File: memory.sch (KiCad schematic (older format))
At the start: 9 parts, among them U5 IS42S16400J-xC

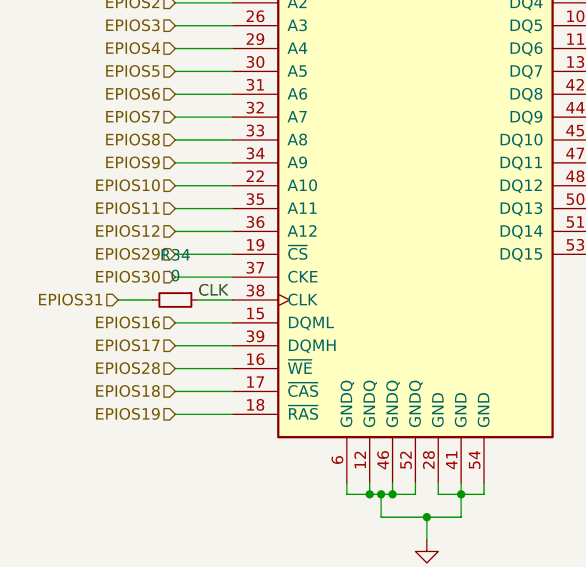
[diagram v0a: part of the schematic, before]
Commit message: updates
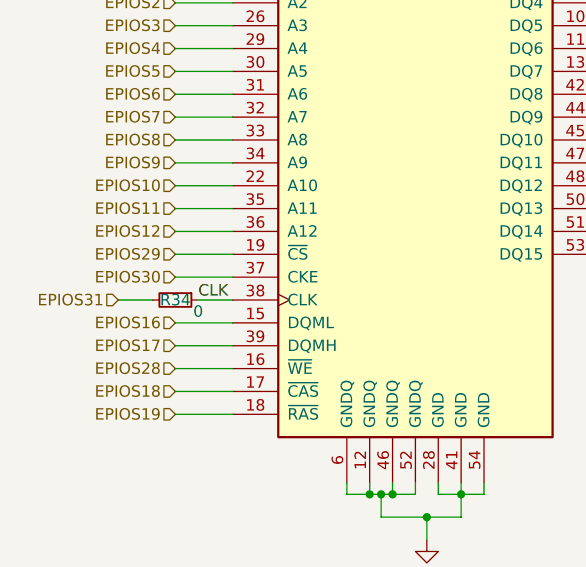
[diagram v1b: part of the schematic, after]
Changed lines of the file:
@@
 EESchema Schematic File Version 4
+LIBS:Raptor2000-cache
 EELAYER 29 0
 EELAYER END
 $Descr A4 11693 8268
 encoding utf-8
-Sheet 10 4
+Sheet 4 4
 Title ""
 Date ""
@@
 U 1 1 5CAC59FE
 P 4750 4050
-F 0 "R34" V 4554 4050 50  0000 C CNN
-F 1 "0" V 4645 4050 50  0000 C CNN
+F 0 "R34" V 4750 4050 50  0000 C CNN
+F 1 "0" V 4800 4150 50  0000 C CNN
 F 2 "Resistor_SMD:R_0603_1608Metric" H 4750 4050 50  0001 C CNN
 F 3 "~" H 4750 4050 50  0001 C CNN

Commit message: added nand flash, removed sd card. finished rtc circuit. added leds
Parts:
- added C14: 0.1, symbol Device:C
- added R4: 10k, symbol Device:R_Small
- added U3: TC58CVG2S0HRAIG, symbol Exodus_Peripherals:TC58CVG2S0HRAIG
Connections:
- net labels added: EPIOS[0..31], FLASH_DAT0, FLASH_DAT1, FLASH_DAT2, FLASH_DAT3, FLASH_SCLK, ~FLASH_CS
- wire segments 104 -> 119
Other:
- moved on the sheet: R34
